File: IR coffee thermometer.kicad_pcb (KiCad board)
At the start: 2 copper layers, 35 x 35 mm, 37 parts, among them J2 USB_C_Receptacle_USB2.0_16P, U1 ESP32-C3FH4, U3 AMS1117, X1 40MHz, 15pF

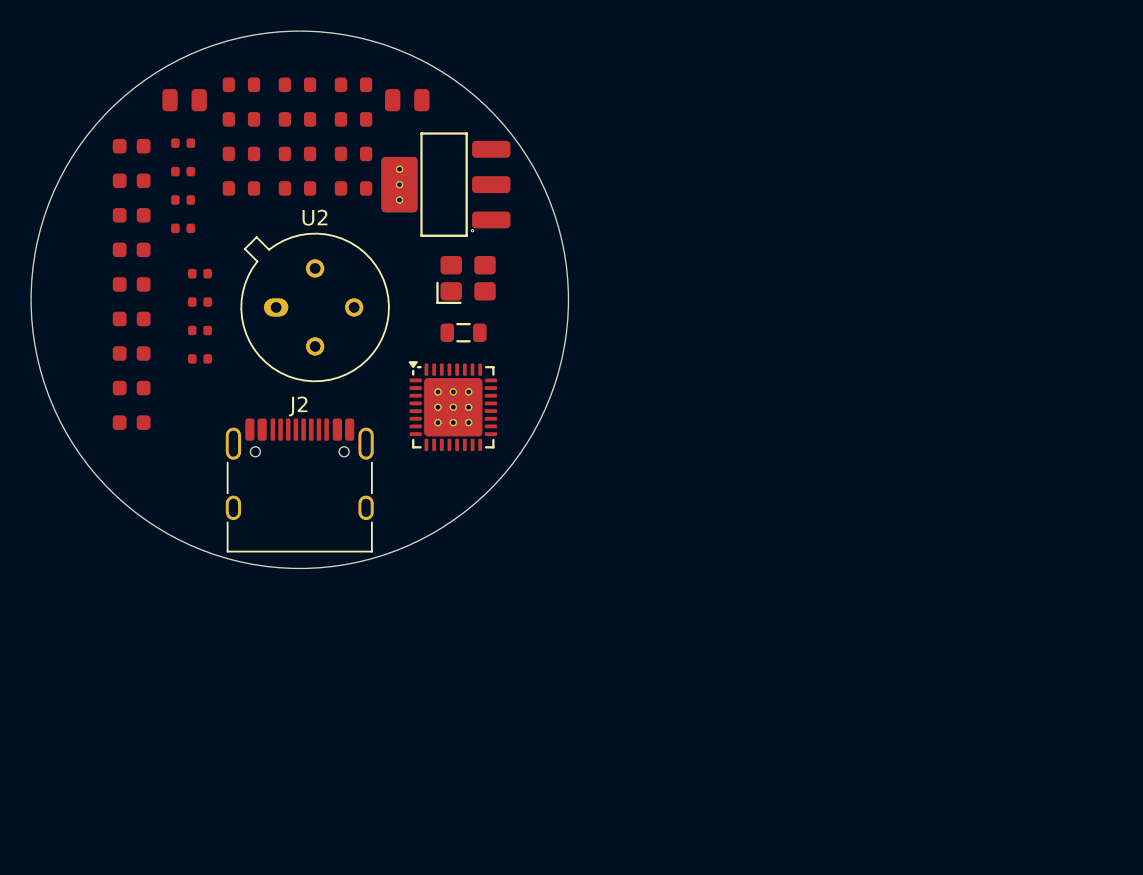
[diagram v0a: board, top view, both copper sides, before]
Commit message: schematic complete
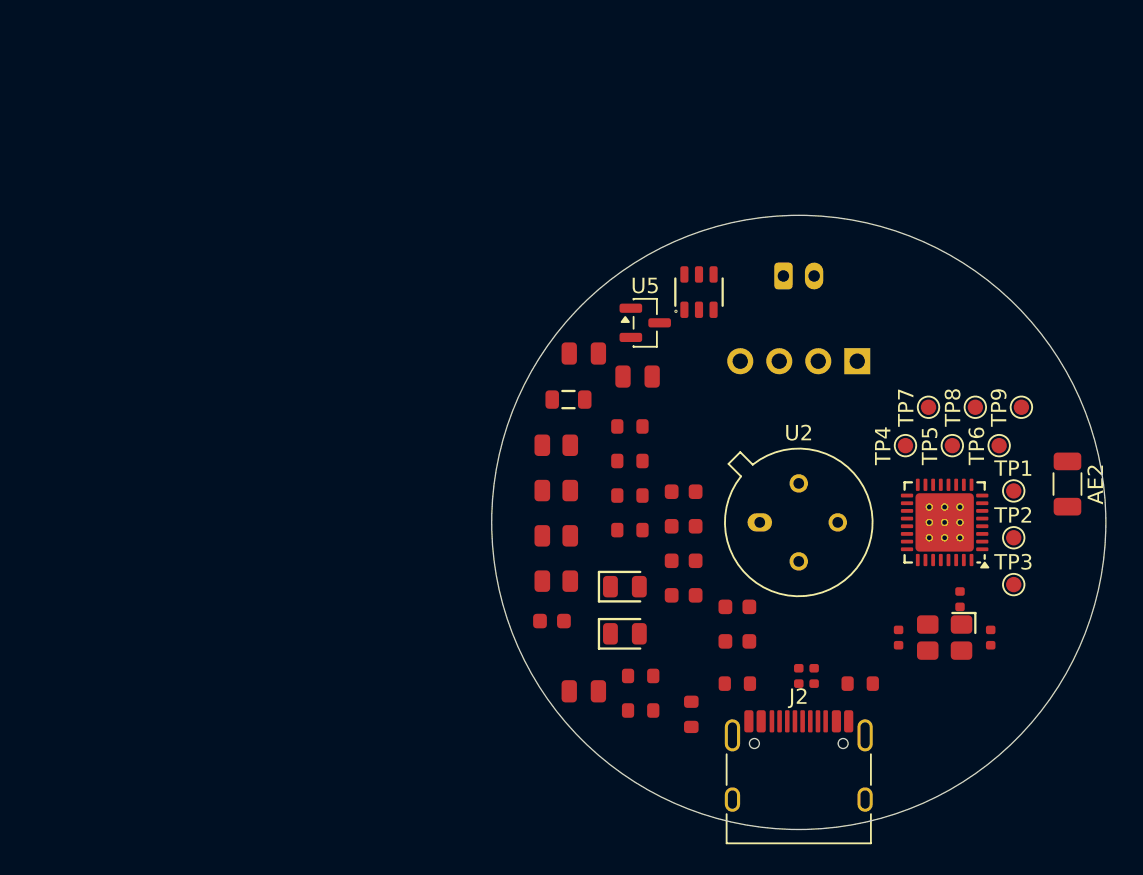
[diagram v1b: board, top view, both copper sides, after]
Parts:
- removed C14: 1.5pF, PCM_JLCPCB:C_0402
- removed C15: 100pF, PCM_JLCPCB:C_0402
- removed C6, C7, C8: 100nF, PCM_JLCPCB:C_0603
- removed R6, R7, R8, R9: 0Ω, PCM_JLCPCB:R_0603
- removed U3: AMS1117, PCM_JLCPCB:SOT-223-3_L6.5-W3.4-P2.30-LS7.0-BR
- added AE2: Antenna_Chip, Capacitor_SMD:C_1206_3216Metric, F.Cu at (167.5, 98.5)
- added C17: 10uF, PCM_JLCPCB:C_0805, F.Cu at (136.0, 90.0)
- added D1: Green, PCM_JLCPCB:D_0805, F.Cu at (138.7, 105.2)
- added D2: Red, PCM_JLCPCB:D_0805, F.Cu at (138.7, 108.3)
- added J1: Conn_01x02_Pin, Connector_JST:JST_PH_B2B-PH-K_1x02_P2.00mm_Vertical, B.Cu at (149.0, 85.0)
- added J3: Conn_01x04_Pin, Connector_PinSocket_2.54mm:PinSocket_1x04_P2.54mm_Vertical, B.Cu at (153.8, 90.5)
- added R10: 510Ω, PCM_JLCPCB:R_0603, F.Cu at (139.0, 99.2)
- added R11: 360Ω, PCM_JLCPCB:R_0603, F.Cu at (139.0, 101.5)
- added R12: 10kΩ, PCM_JLCPCB:R_0805, F.Cu at (134.2, 96.0)
- added R13: 10kΩ, PCM_JLCPCB:R_0805, F.Cu at (134.2, 98.9)
- added R14: 10kΩ, PCM_JLCPCB:R_0805, F.Cu at (134.2, 101.9)
- added REF**: SSD1306 I2C, MyLib:SSD1306 I2C, B.Cu at (150.0, 102.0)
- added TP1: TestPoint, TestPoint:TestPoint_Pad_D1.0mm, F.Cu at (164.0, 99.0)
- added TP2: TestPoint, TestPoint:TestPoint_Pad_D1.0mm, F.Cu at (164.0, 102.0)
- added TP3: TestPoint, TestPoint:TestPoint_Pad_D1.0mm, F.Cu at (164.0, 105.0)
- added TP4: TestPoint, TestPoint:TestPoint_Pad_D1.0mm, F.Cu at (156.9, 96.0)
- added TP5: TestPoint, TestPoint:TestPoint_Pad_D1.0mm, F.Cu at (160.0, 96.0)
- added TP6: TestPoint, TestPoint:TestPoint_Pad_D1.0mm, F.Cu at (163.1, 96.0)
- added TP7: TestPoint, TestPoint:TestPoint_Pad_D1.0mm, F.Cu at (158.4, 93.5)
- added TP8: TestPoint, TestPoint:TestPoint_Pad_D1.0mm, F.Cu at (161.5, 93.5)
- added TP9: TestPoint, TestPoint:TestPoint_Pad_D1.0mm, F.Cu at (164.5, 93.5)
- added U4: TP4057, PCM_JLCPCB:SOT-23-6_L2.9-W1.6-P0.95-LS2.8-BL, F.Cu at (143.5, 86.0)
- added U5: MCP1700x-330xxTT, Package_TO_SOT_SMD:SOT-23, F.Cu at (140.0, 88.0)
- C13: value 1.5pF -> 100nF; footprint PCM_JLCPCB:C_0402 -> PCM_JLCPCB:C_0603
- R15: value 0Ω -> 10kΩ; footprint PCM_JLCPCB:R_0603 -> PCM_JLCPCB:R_0805
- moved C11 60.7 mm to (162.5, 108.5), turned to -90 degrees
- moved C10 56.6 mm to (156.5, 108.5), turned to 90 degrees
- moved R2 53.1 mm to (160.5, 106.0), turned to 90 degrees
- moved C5 46.5 mm to (136.0, 112.0)
- moved R1 46.5 mm to (139.7, 111.0)
- moved R3 46.5 mm to (139.7, 113.2)
- moved R34 46.1 mm to (154.0, 111.5)
- moved R16 45.0 mm to (150.0, 111.0), turned to 90 degrees
- moved R17 45.0 mm to (151.0, 111.0), turned to 90 degrees
- moved R32 44.6 mm to (143.0, 113.5), turned to 90 degrees
- moved R33 42.6 mm to (146.0, 111.5), turned to 180 degrees
- moved C1 42.4 mm to (142.5, 99.0)
- moved C2 42.4 mm to (142.5, 101.2)
- moved C3 42.4 mm to (142.5, 103.5)
- moved C4 42.4 mm to (142.5, 105.8)
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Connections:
- net /CS_SR renamed Net-(J4-Pin_2)
- C13 pad 1: Net-(U1-LNA_IN) -> +3V3
- C16 pad 1: +5V -> VBAT
- R1 pad 1: unconnected-(R1-Pad1) -> Net-(R1-Pad1)
- R15 pad 2: Net-(U1-GPIO9) -> GND
- R32 pad 2: +5V -> VBUS
- R4 pad 1: /MISO -> /SCK
- R4 pad 2: Net-(U1-GPIO2) -> Net-(U1-GPIO10)
- R5 pad 1: /CS_ACC -> /SDA
- R5 pad 2: Net-(U1-GPIO10) -> Net-(U1-GPIO3)
- U1 pad 1: Net-(U1-LNA_IN) -> Net-(AE2-PCB_Trace)
- U1 pad 12: Net-(U1-MTCK) -> unconnected-(U1-MTCK-Pad12)
- U1 pad 13: Net-(U1-MTDO) -> unconnected-(U1-MTDO-Pad13)
- U1 pad 15: Net-(U1-GPIO9) -> Net-(J4-Pin_1)
- U1 pad 21: unconnected-(U1-SPICS0-Pad21) -> Net-(U1-SPICS0)
- U1 pad 22: unconnected-(U1-SPICLK-Pad22) -> Net-(U1-SPICLK)
- U1 pad 23: unconnected-(U1-SPID-Pad23) -> Net-(U1-SPID)
- U1 pad 24: unconnected-(U1-SPIQ-Pad24) -> Net-(U1-SPIQ)
- U1 pad 27: unconnected-(U1-U0RXD-Pad27) -> Net-(U1-U0RXD)
- U2 pad 1: unconnected-(U2-SCL/Vz-Pad1) -> /SCK
- U2 pad 3: unconnected-(U2-VDD-Pad3) -> +3V3
- U2 pad 4: unconnected-(U2-SDA/PWM-Pad4) -> /SDA
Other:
- board size 35 x 35 mm -> 40 x 40 mm

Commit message: schematic complete
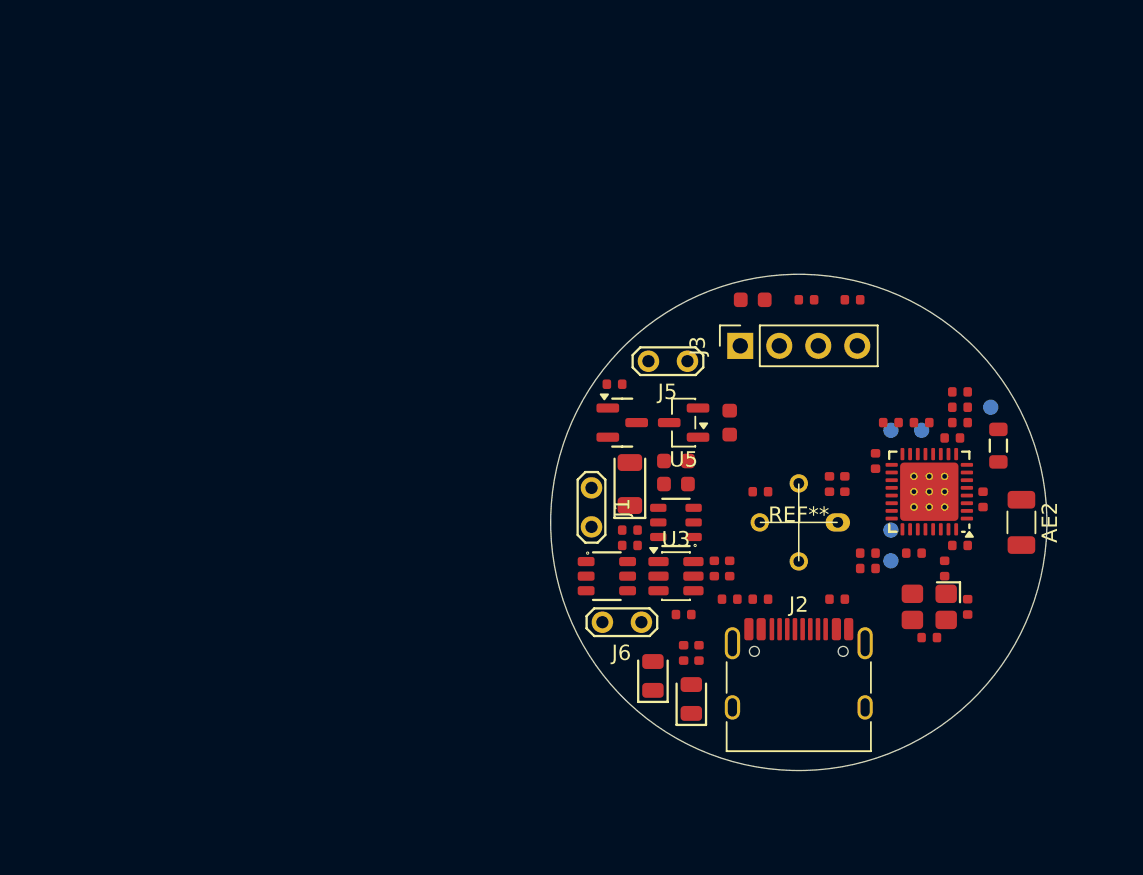
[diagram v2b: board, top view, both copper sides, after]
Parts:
- removed C12, C13: 100nF, PCM_JLCPCB:C_0603
- removed C16, C17: 10uF, PCM_JLCPCB:C_0805
- removed C9: 1uF, PCM_JLCPCB:C_0603
- removed R32: 0Ω, PCM_JLCPCB:R_0603
- removed R33, R34: 5.1kΩ, PCM_JLCPCB:R_0603
- removed TP6, TP7, TP8, TP9: TestPoint, TestPoint:TestPoint_Pad_D1.0mm
- added C15: 100nF, PCM_JLCPCB:C_0402, F.Cu at (160.5, 94.5)
- added C19: 100nF, PCM_JLCPCB:C_0402, F.Cu at (160.0, 95.5)
- added C20: 100nF, PCM_JLCPCB:C_0402, F.Cu at (160.5, 102.5)
- added C21: 100nF, PCM_JLCPCB:C_0402, F.Cu at (155.0, 97.0)
- added C22: 100nF, PCM_JLCPCB:C_0402, F.Cu at (147.5, 99.0)
- added C6: 100nF, PCM_JLCPCB:C_0402, F.Cu at (144.5, 104.0)
- added D3: 1N4001W, PCM_JLCPCB:D_SOD-123FL, F.Cu at (139.0, 98.5)
- added J5: Conn_01x02_Pin, TestPoint:TestPoint_2Pads_Pitch2.54mm_Drill0.8mm, F.Cu at (142.8, 90.5)
- added J6: Conn_01x02_Pin, TestPoint:TestPoint_2Pads_Pitch2.54mm_Drill0.8mm, F.Cu at (139.8, 107.5)
- added Q1: HJ8205, PCM_JLCPCB:SOT-23-6_L2.9-W1.6-P0.95-LS2.8-BR, F.Cu at (137.5, 104.5)
- added Q2: HL2305, PCM_JLCPCB:Q_SOT-23, F.Cu at (138.5, 94.5)
- added R18: 0Ω, PCM_JLCPCB:R_0402, F.Cu at (145.5, 106.0)
- added R19: 0Ω, PCM_JLCPCB:R_0402, F.Cu at (152.0, 98.5)
- added R20: 0Ω, PCM_JLCPCB:R_0402, F.Cu at (153.0, 98.5)
- added R21: 470Ω, PCM_JLCPCB:R_0402, F.Cu at (157.5, 103.0)
- added R22: 470Ω, PCM_JLCPCB:R_0402, F.Cu at (145.5, 104.0)
- added R6: 330Ω, PCM_JLCPCB:R_0402, F.Cu at (142.5, 109.5)
- added R7: 2kΩ, PCM_JLCPCB:R_0402, F.Cu at (142.5, 107.0)
- added R8: 10kΩ, PCM_JLCPCB:R_0402, F.Cu at (138.0, 92.0)
- added R9: 0Ω, PCM_JLCPCB:R_0402, F.Cu at (139.0, 101.5)
- added U3: DW01A, Package_TO_SOT_SMD:SOT-23-6, F.Cu at (142.0, 104.5)
- C1, C3, C4: value 100nF -> 10uF
- C2: value 100nF -> 1uF; footprint PCM_JLCPCB:C_0603 -> PCM_JLCPCB:C_0402
- C5: footprint PCM_JLCPCB:C_0805 -> PCM_JLCPCB:C_0603
- J1: footprint Connector_JST:JST_PH_B2B-PH-K_1x02_P2.00mm_Vertical -> TestPoint:TestPoint_2Pads_Pitch2.54mm_Drill0.8mm; moved to F.Cu
- J3, REF**: moved to F.Cu
- R1: value 470Ω -> 510Ω; footprint PCM_JLCPCB:R_0603 -> PCM_JLCPCB:R_0402
- R10: value 510Ω -> 1kΩ; footprint PCM_JLCPCB:R_0603 -> PCM_JLCPCB:R_0402
- R11: value 360Ω -> 10kΩ; footprint PCM_JLCPCB:R_0603 -> PCM_JLCPCB:R_0402
- R12, R13: footprint PCM_JLCPCB:R_0805 -> PCM_JLCPCB:R_0402
- R14, R15: value 10kΩ -> 5.1kΩ; footprint PCM_JLCPCB:R_0805 -> PCM_JLCPCB:R_0402
- R3: value 1kΩ -> 4.7kΩ; footprint PCM_JLCPCB:R_0603 -> PCM_JLCPCB:R_0402
- R4: value 0Ω -> 4.7kΩ; footprint PCM_JLCPCB:R_0603 -> PCM_JLCPCB:R_0402
- R5: value 0Ω -> 10kΩ; footprint PCM_JLCPCB:R_0603 -> PCM_JLCPCB:R_0402
- TP1, TP2, TP3, TP4, TP5, U2: moved to B.Cu
- moved R3 30.1 mm to (153.5, 86.5)
- moved FB1 28.2 mm to (163.0, 96.0), turned to 90 degrees
- moved C5 27.8 mm to (147.0, 86.5), turned to 180 degrees
- moved R13 27.1 mm to (160.5, 92.5)
- moved R10 22.3 mm to (160.5, 93.5), turned to 180 degrees
- moved C2 19.6 mm to (162.0, 99.5), turned to 90 degrees
- moved R5 19.2 mm to (158.0, 94.5)
- moved J1 18.6 mm to (136.5, 98.8), turned to -90 degrees
- moved R11 18.4 mm to (156.0, 94.5), turned to 180 degrees
- moved R15 18.3 mm to (152.5, 106.0)
- moved U4 15.1 mm to (142.0, 101.0), turned to 90 degrees
- moved R4 14.2 mm to (150.5, 86.5)
- moved R14 13.9 mm to (147.5, 106.0), turned to 180 degrees
- moved TP3 11.7 mm to (158.0, 95.0)
- moved C4 11.6 mm to (145.5, 94.5), turned to -90 degrees
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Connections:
- C1 pad 1: +3V3 -> Net-(J5-Pin_1)
- C2 pad 1: +3V3 -> 3V3_FILT
- C3 pad 1: +3V3 -> VBUS
- J1 pad 2: GND -> Net-(J1-Pin_2)
- R1 pad 1: Net-(R1-Pad1) -> VBUS
- R1 pad 2: Net-(U1-U0TXD) -> Net-(D2-Pad2)
- R10 pad 1: VBUS -> Net-(U1-CHIP_EN)
- R10 pad 2: Net-(D2-Pad2) -> +3V3
- R11 pad 1: VBUS -> +3V3
- R11 pad 2: Net-(D1-Pad2) -> Net-(U1-GPIO9)
- R14 pad 1: +3V3 -> Net-(J2-CC1)
- R14 pad 2: Net-(U1-GPIO8) -> GND
- R15 pad 1: Net-(J4-Pin_2) -> Net-(J2-CC2)
- R3 pad 1: Net-(U1-CHIP_EN) -> +3V3
- R3 pad 2: +3V3 -> /SDA
- R4 pad 1: /SCK -> +3V3
- R4 pad 2: Net-(U1-GPIO10) -> /SCK
- R5 pad 1: /SDA -> +3V3
- R5 pad 2: Net-(U1-GPIO3) -> Net-(U1-GPIO8)
- TP1 pad 1: Net-(R1-Pad1) -> Net-(R21-Pad1)
- TP4 pad 1: Net-(J4-Pin_1) -> Net-(U1-GPIO9)
- U1 pad 15: Net-(J4-Pin_1) -> Net-(U1-GPIO9)
- U1 pad 21: Net-(U1-SPICS0) -> unconnected-(U1-SPICS0-Pad21)
- U1 pad 22: Net-(U1-SPICLK) -> unconnected-(U1-SPICLK-Pad22)
- U1 pad 23: Net-(U1-SPID) -> unconnected-(U1-SPID-Pad23)
- U1 pad 24: Net-(U1-SPIQ) -> unconnected-(U1-SPIQ-Pad24)
- U2 pad 2: (no net) -> /SDA
- U2 pad 4: /SDA -> GND
- U5 pad 3: VBAT -> Net-(J5-Pin_1)
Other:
- board size 40 x 40 mm -> 32.3 x 32.3 mm

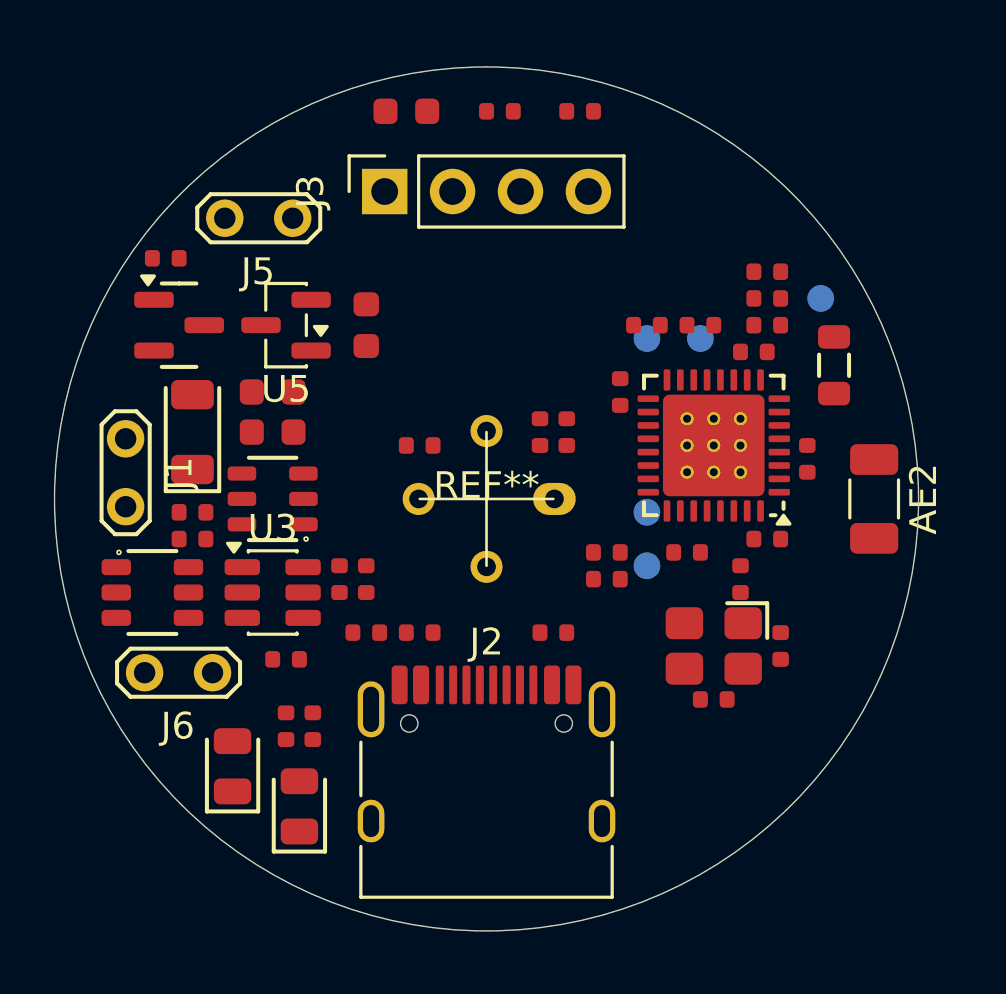
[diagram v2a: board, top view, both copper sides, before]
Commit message: routing complete
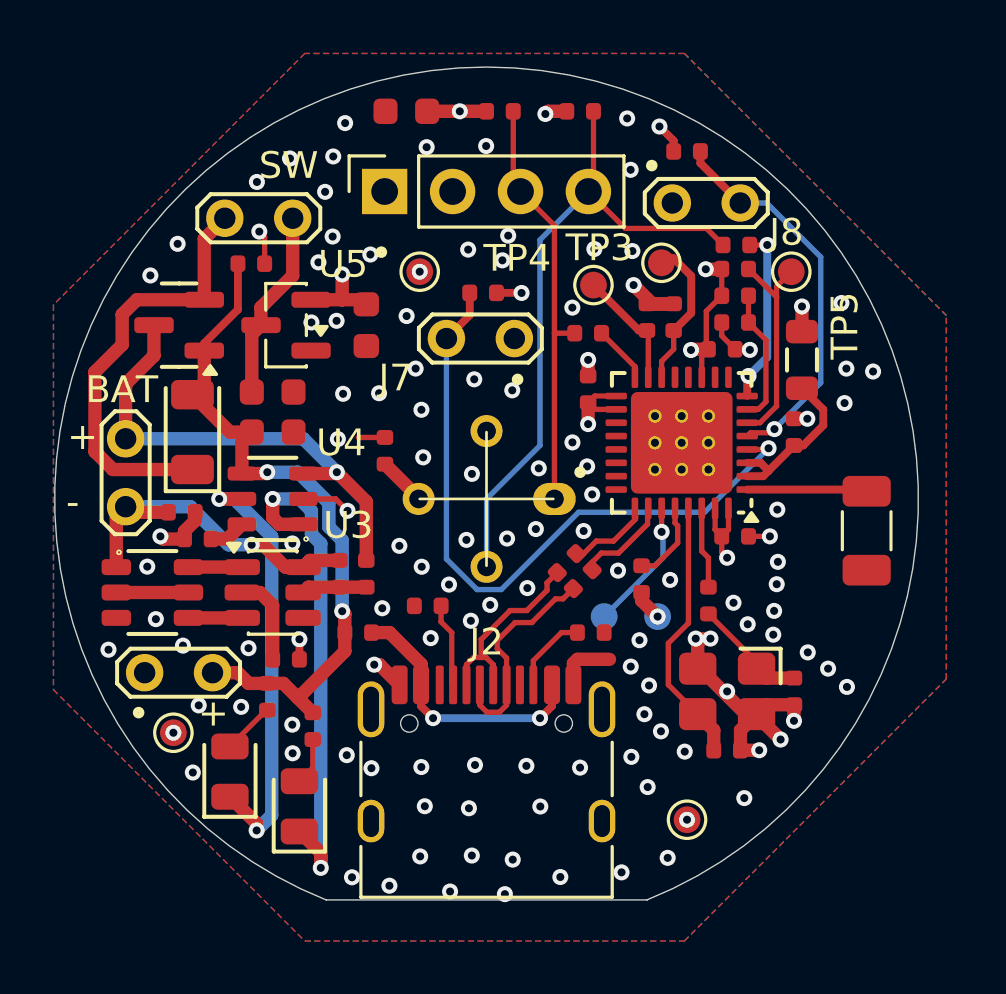
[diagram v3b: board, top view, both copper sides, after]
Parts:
- removed Q1: HJ8205, PCM_JLCPCB:SOT-23-6_L2.9-W1.6-P0.95-LS2.8-BR
- added J7: Conn_01x02_Pin, TestPoint:TestPoint_2Pads_Pitch2.54mm_Drill0.8mm, F.Cu at (148.5, 95.0)
- added J8: Conn_01x02_Pin, TestPoint:TestPoint_2Pads_Pitch2.54mm_Drill0.8mm, F.Cu at (159.5, 89.9)
- added Q3: HJ8205, PCM_JLCPCB:SOT-23-6_L2.9-W1.6-P0.95-LS2.8-BR, F.Cu at (137.5, 104.5)
- added R23: 10kΩ, PCM_JLCPCB:R_0402, F.Cu at (149.9, 93.3)
- added R24: 10kΩ, PCM_JLCPCB:R_0402, F.Cu at (157.5, 88.0)
- added TP6: TestPoint, TestPoint:TestPoint_Pad_D1.0mm, F.Cu at (147.5, 92.5)
- added TP7: TestPoint, TestPoint:TestPoint_Pad_D1.0mm, F.Cu at (138.3, 109.7)
- added TP8: TestPoint, TestPoint:TestPoint_Pad_D1.0mm, F.Cu at (157.5, 113.0)
- TP3, TP4, TP5: moved to F.Cu
- moved R19 10.1 mm to (159.3, 91.5), turned to 0 degrees
- moved TP2 4.22 mm to (154.4, 105.4)
- moved R20 3.79 mm to (153.8, 94.8), turned to 0 degrees
- moved R8 3.21 mm to (141.2, 92.2)
- moved TP3 3.19 mm to (156.5, 92.2), turned to 180 degrees
- moved TP4 2.83 mm to (154.0, 93.0)
- moved R21 1.97 mm to (155.8, 104.0), turned to 90 degrees
- moved C10 1.96 mm to (159.0, 110.4)
- moved TP1 1.94 mm to (156.4, 105.4)
- moved C11 1.77 mm to (161.5, 108.2)
- moved X1 1.77 mm to (159.0, 108.2)
- moved R16 1.55 mm to (153.0, 103.4), turned to 45 degrees
- moved TP5 1.49 mm to (161.4, 92.5)
- moved R2 1.44 mm to (158.3, 104.8)
- moved R15 1.40 mm to (153.9, 106.0)
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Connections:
- net Net-(U1-GPIO18/USB_D-) renamed /USB_ESP_N
- net Net-(U1-GPIO19/USB_D+) renamed /USB_ESP_P
- AE2 pad 1: GND -> unconnected-(AE2-FEED-Pad1)
- U1 pad 4: unconnected-(U1-GPIO0/XTAL_32K_P-Pad4) -> Net-(J7-Pin_1)
- U1 pad 5: unconnected-(U1-GPIO1/XTAL_32K_N-Pad5) -> Net-(J8-Pin_1)
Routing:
- net VBUS: track 0.00 -> 26.5 mm, vias 0 -> 2
- net Net-(J7-Pin_1): track 0.00 -> 25.8 mm, vias 0 -> 1
- net +3V3: track 0.00 -> 25.8 mm, vias 0 -> 11
- net /SDA: track 0.00 -> 24.6 mm
- net GND: track 0.00 -> 24.5 mm, vias 0 -> 121
- net Net-(U4-CHRG): track 0.00 -> 18.8 mm, vias 0 -> 2
- net VBAT: track 0.00 -> 18.1 mm, vias 0 -> 1
- net Net-(U4-STDBY): track 0.00 -> 16.3 mm, vias 0 -> 2
- net Net-(J5-Pin_2): track 0.00 -> 16.1 mm
- net /SCK: track 0.00 -> 15.9 mm
- net Net-(J8-Pin_1): track 0.00 -> 14.7 mm, vias 0 -> 1
- net Net-(J1-Pin_2): track 0.00 -> 13.1 mm, vias 0 -> 1
- net Net-(U1-XTAL_N): track 0.00 -> 10.1 mm
- net Net-(J2-VBUS-PadA4): track 0.00 -> 9.98 mm, vias 0 -> 2
- net /USB_P: track 0.00 -> 8.19 mm
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- added copper zone on In2.Cu, net +3V3
- added copper zone on B.Cu, net GND
- added copper zone on F.Cu, net GND
- added copper zone on In1.Cu, net GND
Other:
- board size 32.3 x 32.3 mm -> 32.3 x 31.2 mm
- copper layers 2 -> 4
- board text added: "+"
- board text added: "-"
- board text added: "BAT"
- board text added: "SW"
- board text added: "TX RX"
